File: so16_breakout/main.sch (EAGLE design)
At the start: 5 parts

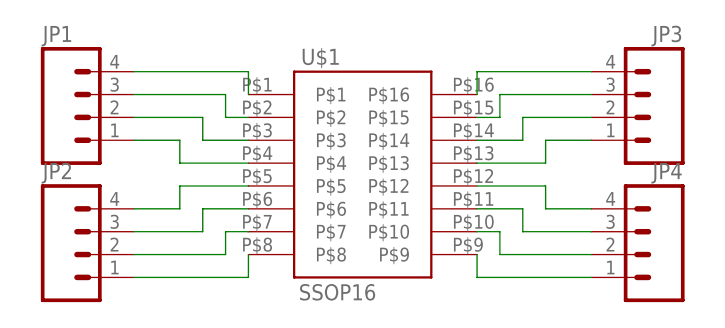
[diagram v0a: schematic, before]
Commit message: [ update ] so16_breakout
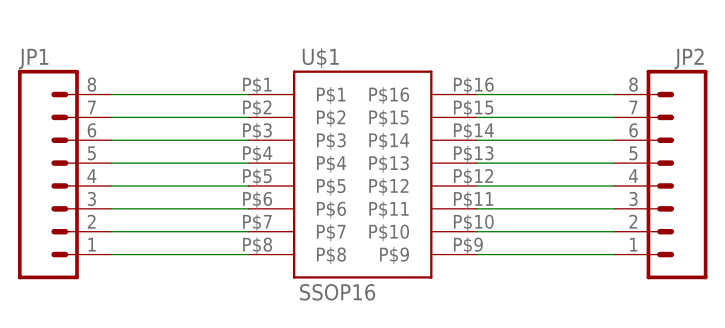
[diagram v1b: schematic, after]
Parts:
- removed JP3, JP4: (no value), SparkFun:M04PTH
- JP1, JP2: device SparkFun:M04PTH -> SparkFun:M08LONGPADS
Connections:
- net N$1: now also JP1.8; no longer JP1.4
- net N$10: now also JP2.7; no longer JP3.3
- net N$11: now also JP2.6; no longer JP3.2
- net N$12: now also JP2.5; no longer JP3.1
- net N$13: now also JP2.4; no longer JP4.4
- net N$14: now also JP2.3; no longer JP4.3
- net N$15: now also JP2.2; no longer JP4.2
- net N$16: now also JP2.1; no longer JP4.1
- net N$2: now also JP1.7; no longer JP1.3
- net N$3: now also JP1.6; no longer JP1.2
- net N$4: now also JP1.5; no longer JP1.1
- net N$5: now also JP1.4; no longer JP2.4
- net N$6: now also JP1.3; no longer JP2.3
- net N$7: now also JP1.2; no longer JP2.2
- net N$8: now also JP1.1; no longer JP2.1
- net N$9: now also JP2.8; no longer JP3.4
